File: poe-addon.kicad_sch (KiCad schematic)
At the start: 16 parts, among them U1 25AA02E48T-I_OT, X1 ARJM11-104, X2 Conn_01x05_Male, X3 Conn_01x05_Male

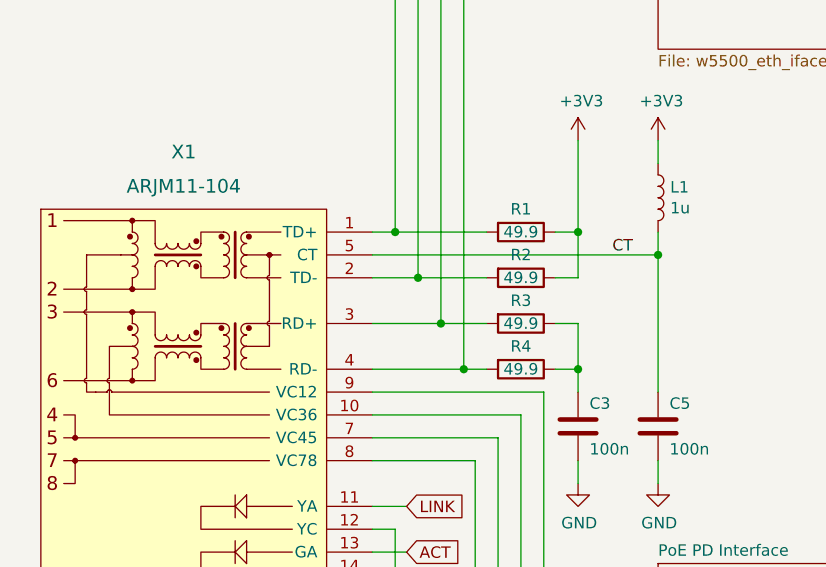
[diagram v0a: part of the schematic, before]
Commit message: Add LCSC part numbers
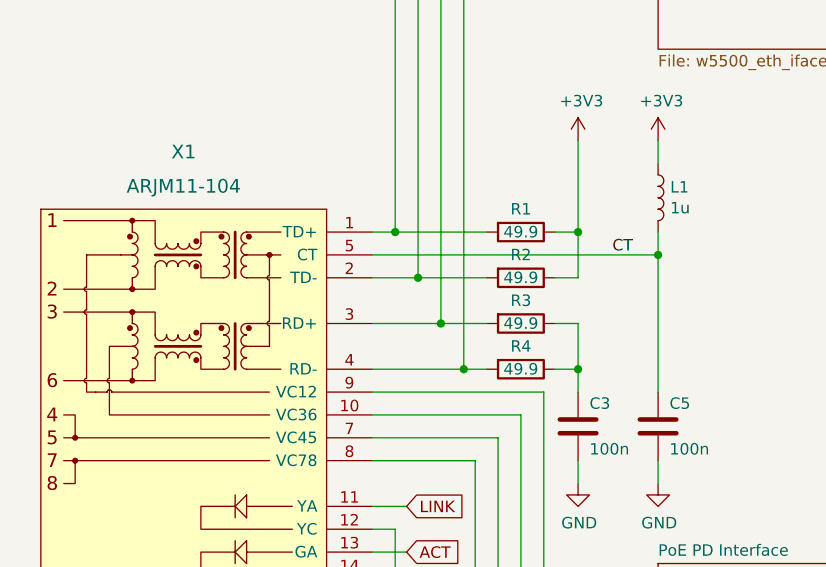
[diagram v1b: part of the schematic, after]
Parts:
- C1, C3, C5: LCSC (none) -> C14663
- C2, C4: LCSC (none) -> C57112
- L1: LCSC (none) -> C1034
- R1, R2, R3, R4: LCSC (none) -> C844569
- U1: LCSC (none) -> C145570
